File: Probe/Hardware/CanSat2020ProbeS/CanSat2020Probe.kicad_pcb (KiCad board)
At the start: 2 copper layers, 35 parts, among them IC1 TESEO-LIV3F, J1 BME280, J2 MPU-9250, J3 Micro_SD_Card, J4 Conn_01x03_Male, J5 Conn_Coaxial, J6 Conn_Coaxial, J7 Conn_01x05_Male, J8 Conn_01x02_Male, SW1 SW_DIP_x01, U1 STM32F411RETx, U2 RFM69HW, U3 LD3985M33R_SOT23, Y1 Crystal

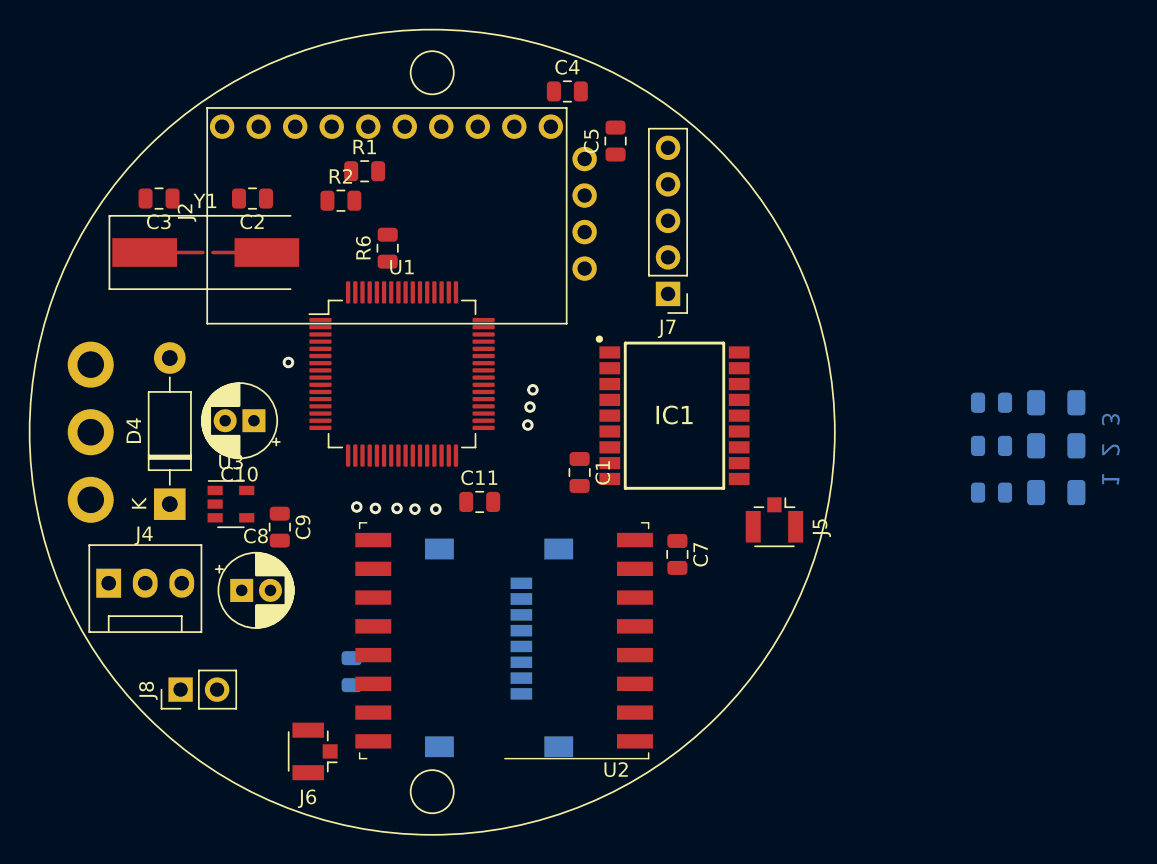
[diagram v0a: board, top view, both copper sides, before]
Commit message: minor changes
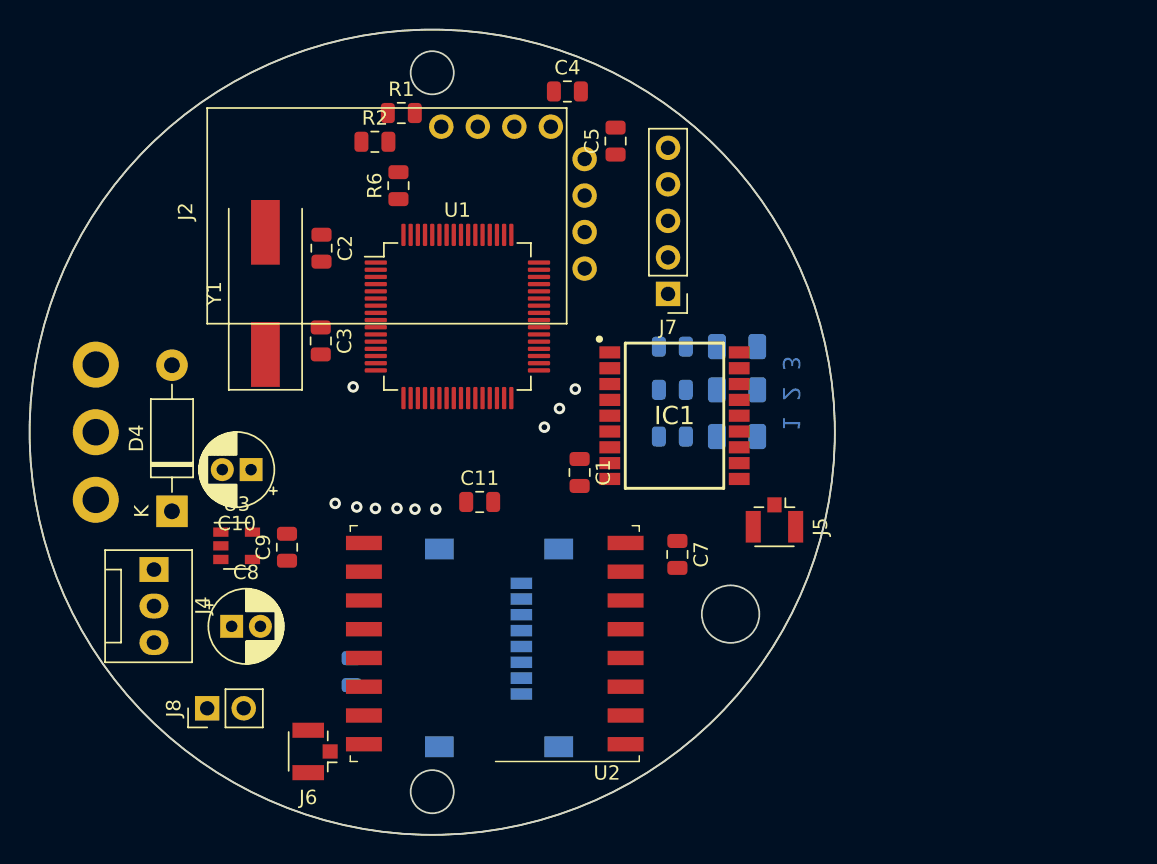
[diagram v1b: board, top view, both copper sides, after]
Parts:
- J2: footprint Switch:MPU-9250 -> Switch:MPU-9250-4pin
- U2: value RFM69HW -> RFM69W
- moved D1 22.5 mm to (171.2, 100.3)
- moved D2 22.5 mm to (171.2, 97.0)
- moved D3 22.5 mm to (171.2, 94.0)
- moved R3 22.5 mm to (166.7, 100.3), turned to 0 degrees
- moved R4 22.5 mm to (166.7, 97.0), turned to 0 degrees
- moved R5 22.5 mm to (166.7, 94.0), turned to 0 degrees
- moved C3 15.0 mm to (142.2, 93.7), turned to 270 degrees
- moved C2 5.91 mm to (142.3, 87.2), turned to 270 degrees
- moved U1 5.55 mm to (151.8, 92.0)
- moved Y1 5.03 mm to (138.4, 90.3), turned to 90 degrees
- moved R1 4.79 mm to (147.8, 77.8)
- moved R2 4.73 mm to (146.0, 79.8)
- moved R6 4.41 mm to (147.7, 82.8)
- moved C10 3.41 mm to (137.4, 102.6)
- moved J4 3.29 mm to (130.7, 109.5), turned to 270 degrees
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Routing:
- net Net-(C3-Pad2): track 4.05 -> 0.00 mm
- net Net-(C2-Pad1): track 3.75 -> 0.00 mm
- net Net-(U2-Pad16): vias 0 -> 1
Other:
- board outline added: 56 x 56 mm
